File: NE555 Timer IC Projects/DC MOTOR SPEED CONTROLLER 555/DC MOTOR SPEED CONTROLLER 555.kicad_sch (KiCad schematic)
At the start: 12 parts, among them M1 Motor_DC, Q1 IRLZ44N, U1 LM555xM

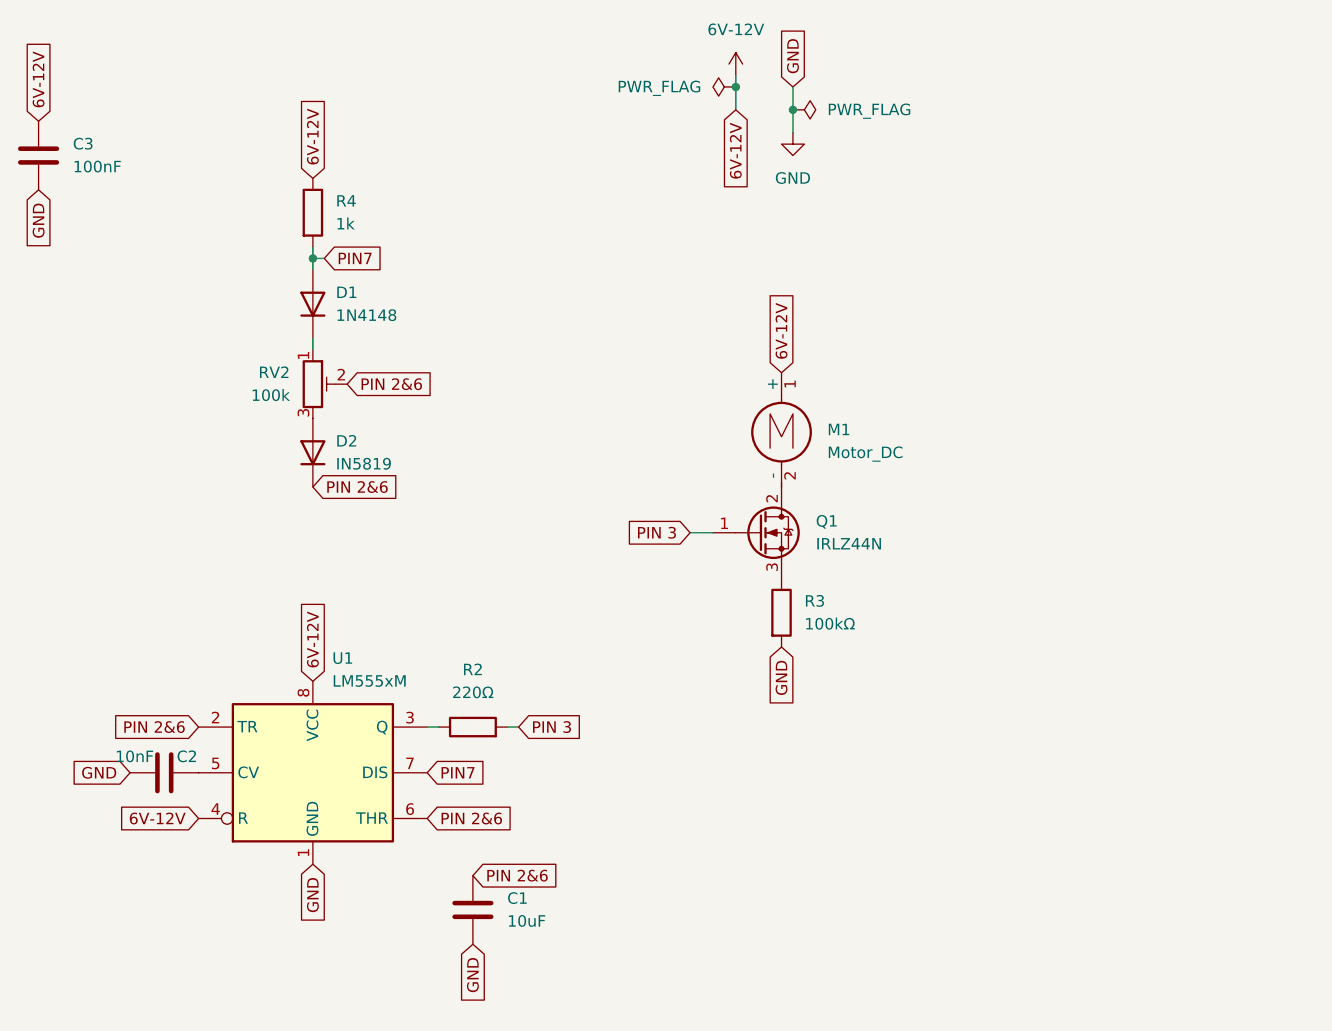
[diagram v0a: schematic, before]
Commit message: Initial Commit
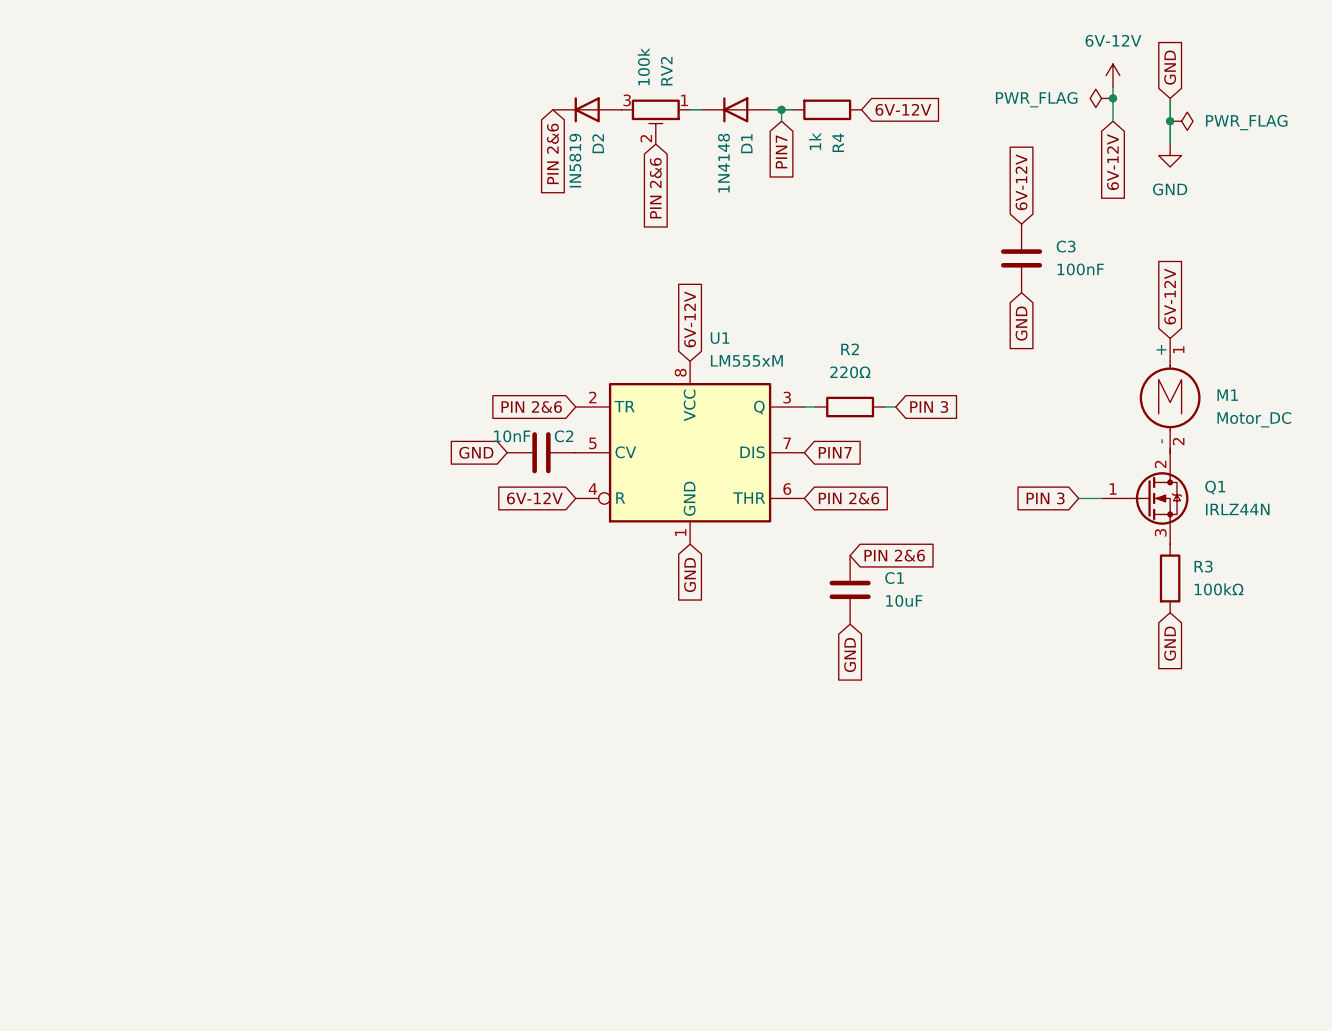
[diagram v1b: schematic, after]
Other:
- moved on the sheet: C1, C2, C3, D1, D2, M1, Q1, R2, R3, R4, RV2, U1
